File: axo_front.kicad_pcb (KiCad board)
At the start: 2 copper layers, 20 x 128.5 mm, 0 parts

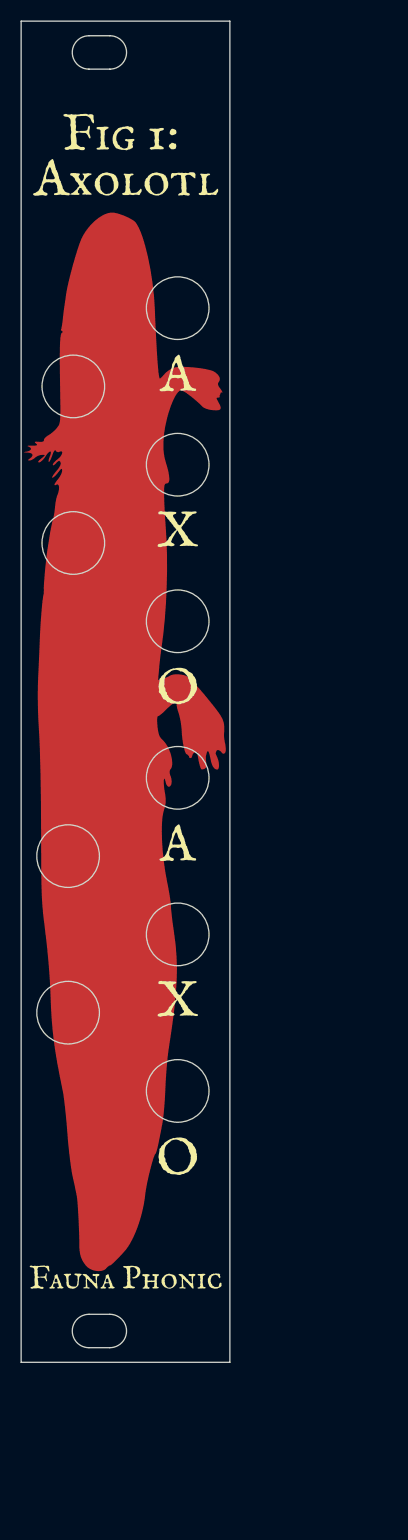
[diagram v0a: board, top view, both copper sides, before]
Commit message: update pcb
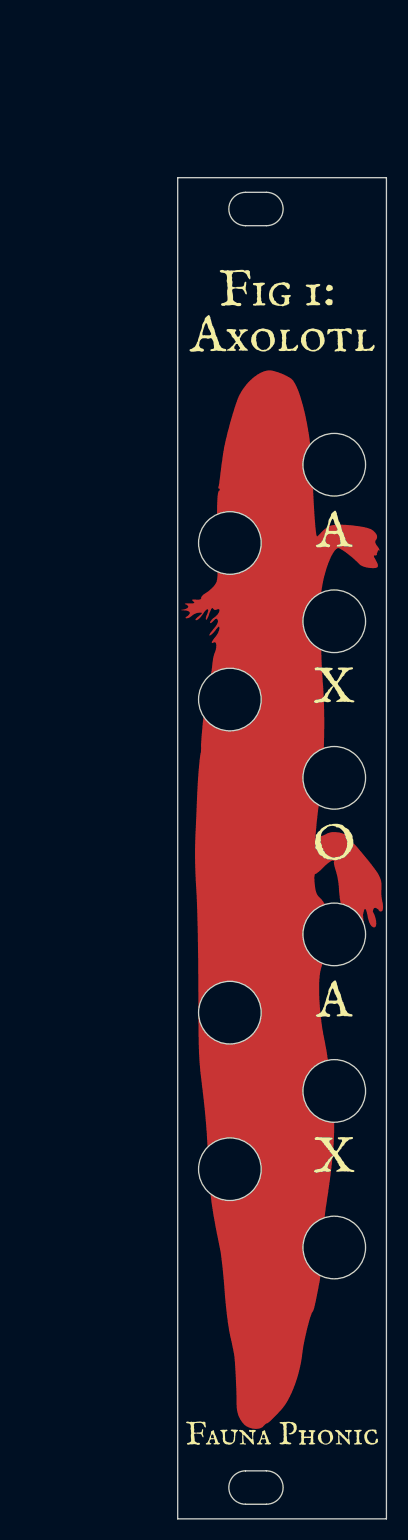
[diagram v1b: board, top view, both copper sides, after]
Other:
- outline, holes or cut-outs redrawn
- board text removed: "AXOLOTL Front Panel - REV 1.0 Pierre Lamot 2024 JLCJLCJLCJLC"
